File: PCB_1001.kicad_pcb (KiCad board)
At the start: 2 copper layers, 26.9 x 30.2 mm, 4 parts, among them SW1 SW_SPST

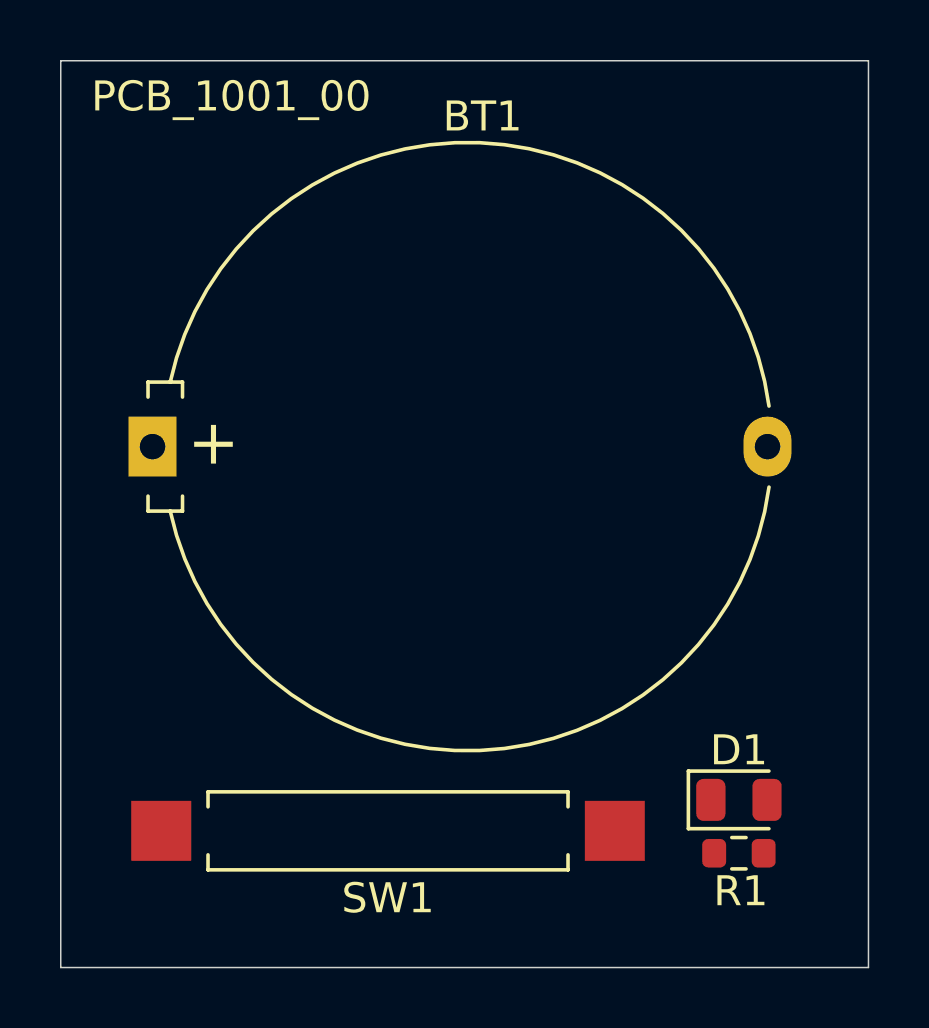
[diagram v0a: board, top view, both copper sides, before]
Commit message: Routing complete
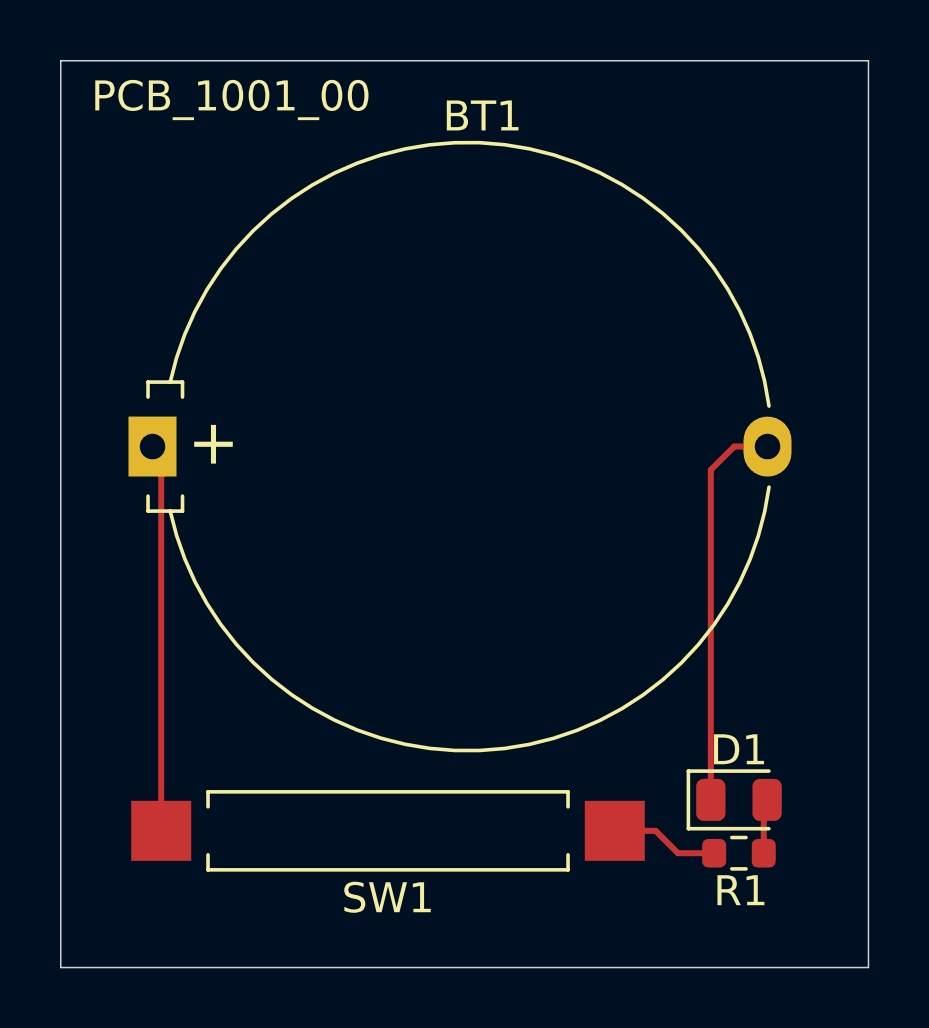
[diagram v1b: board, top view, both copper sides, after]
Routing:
- net Net-(BT1--): track 0.00 -> 13.2 mm
- net Net-(BT1-+): track 0.00 -> 12.9 mm
- net Net-(SW1-B): track 0.00 -> 3.62 mm
- net Net-(D1-A): track 0.00 -> 1.82 mm
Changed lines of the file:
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@@
 		(fp_arc
 			(start 20.68 -1.32)
-			(mid 21.329593 -0.950487)
+			(mid 21.329556 -0.950479)
 			(end 21.59 -0.25)
 			(stroke
@@
 		)
 	)
+	(segment
+		(start 131.873 98.568)
+		(end 131.873 86.049607)
+		(width 0.2)
+		(layer "F.Cu")
+		(net 1)
+	)
+	(segment
+		(start 131.873 86.049607)
+		(end 131.583 85.759607)
+		(width 0.2)
+		(layer "F.Cu")
+		(net 1)
+	)
+	(segment
+		(start 150.1925 97.536)
+		(end 150.1925 86.5355)
+		(width 0.2)
+		(layer "F.Cu")
+		(net 2)
+	)
+	(segment
+		(start 150.1925 86.5355)
+		(end 150.968393 85.759607)
+		(width 0.2)
+		(layer "F.Cu")
+		(net 2)
+	)
+	(segment
+		(start 150.968393 85.759607)
+		(end 152.083 85.759607)
+		(width 0.2)
+		(layer "F.Cu")
+		(net 2)
+	)
+	(segment
+		(start 151.955 99.314)
+		(end 151.955 97.6485)
+		(width 0.2)
+		(layer "F.Cu")
+		(net 3)
+	)
+	(segment
+		(start 151.955 97.6485)
+		(end 152.0675 97.536)
+		(width 0.2)
+		(layer "F.Cu")
+		(net 3)
+	)
+	(segment
+		(start 148.352 98.568)
+		(end 149.098 99.314)
+		(width 0.2)
+		(layer "F.Cu")
+		(net 4)
+	)
+	(segment
+		(start 149.098 99.314)
+		(end 150.305 99.314)
+		(width 0.2)
+		(layer "F.Cu")
+		(net 4)
+	)
+	(segment
+		(start 146.993 98.568)
+		(end 148.352 98.568)
+		(width 0.2)
+		(layer "F.Cu")
+		(net 4)
+	)
 )
